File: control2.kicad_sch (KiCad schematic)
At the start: 16 parts, among them J8 AudioJack3_SwitchTR, J9 AudioJack3_SwitchTR, U10 USBLC6-2SC6, U4 74HC595, U6 74HC595, U7 74HC595, U8 74HC595, U9 USBLC6-2SC6

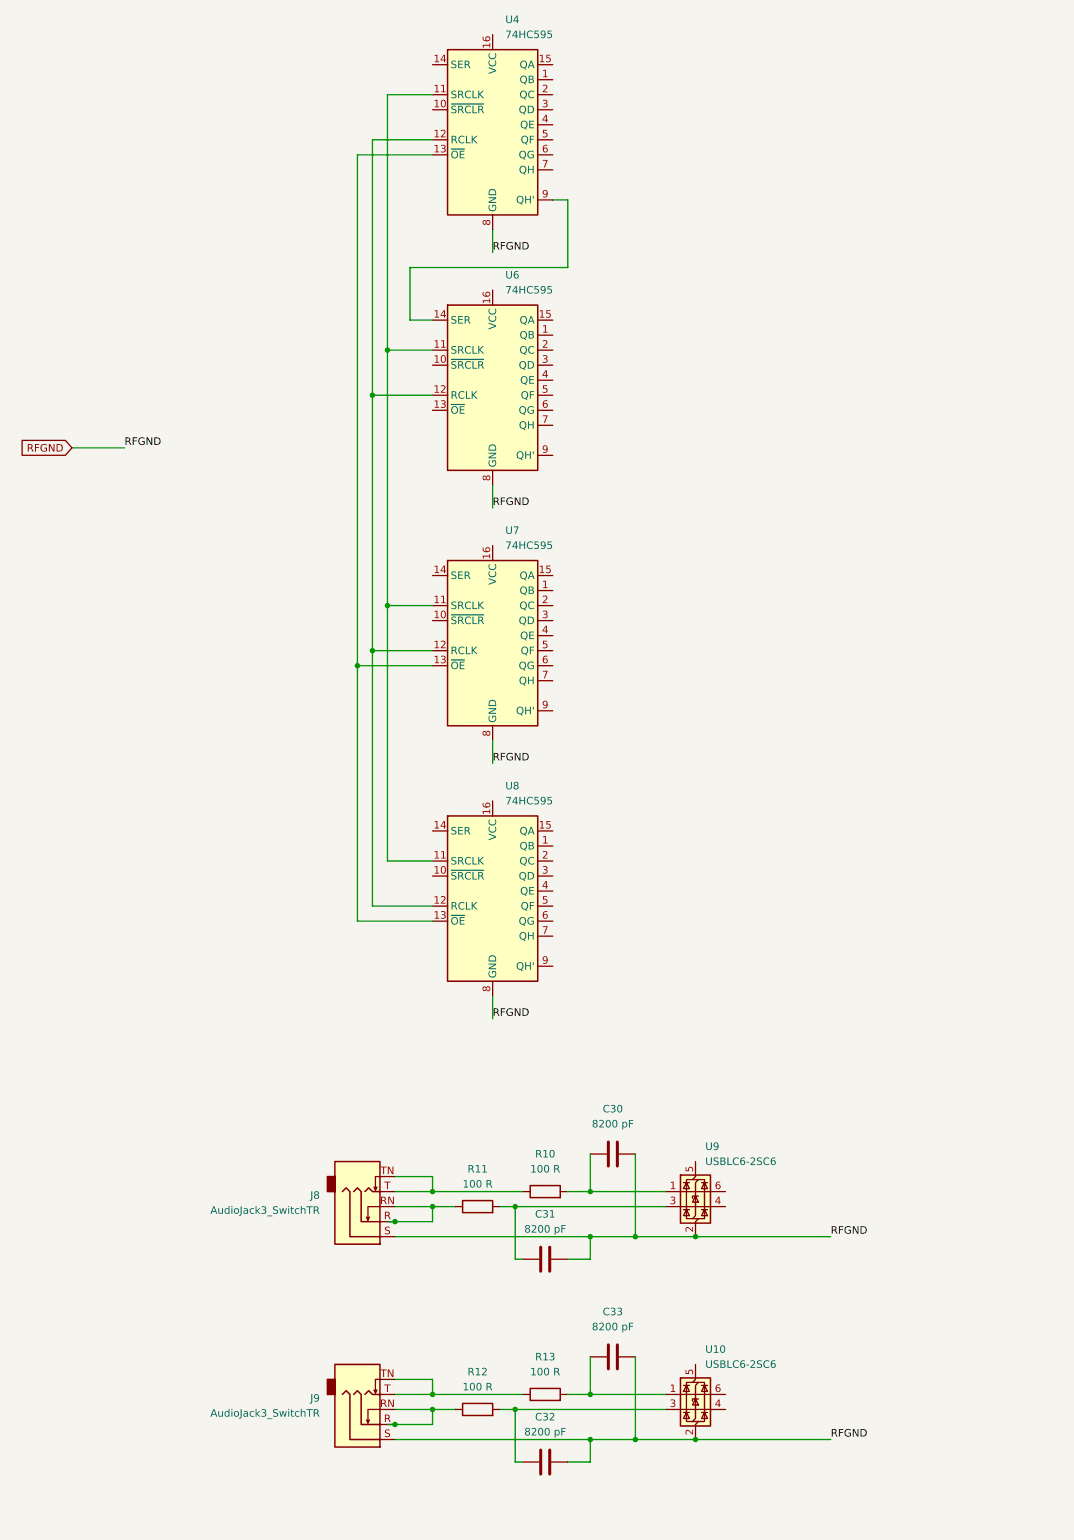
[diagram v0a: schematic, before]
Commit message: Перевёл на иерархические схемы
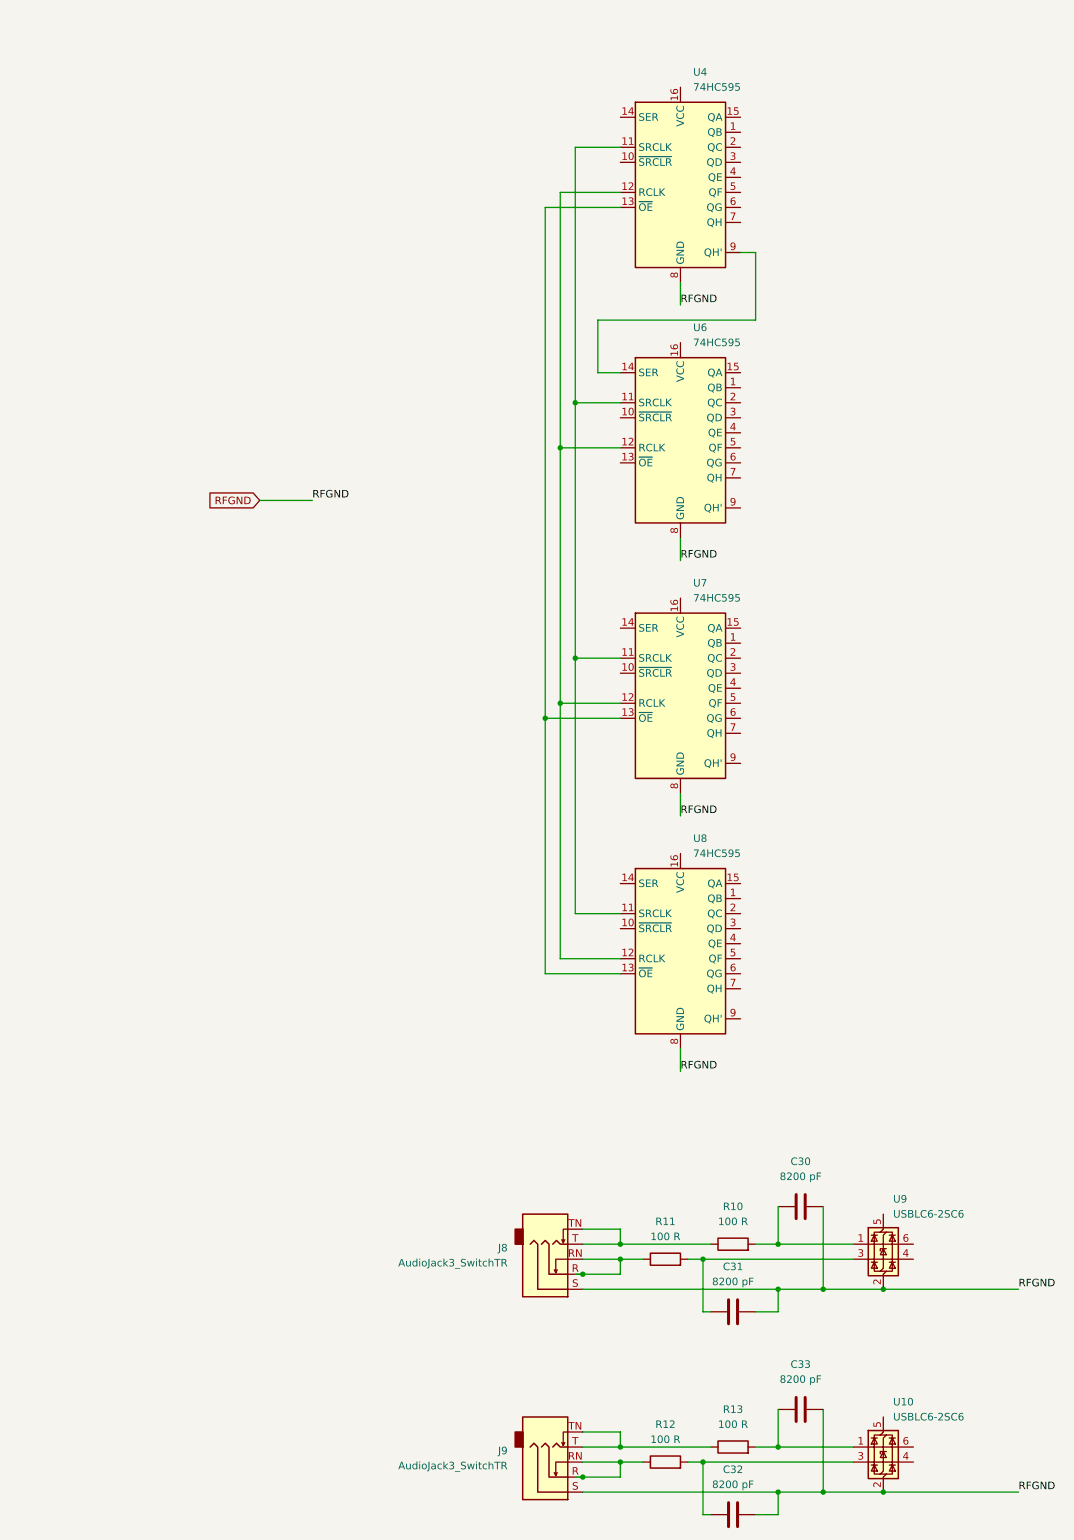
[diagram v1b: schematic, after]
